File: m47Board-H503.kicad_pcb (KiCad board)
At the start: 4 copper layers, 40 x 34 mm, 42 parts, among them J1 USB_C_Receptacle_USB2.0_16P, J3 Conn_01x15_Pin, J4 Conn_01x10_Pin, J5 Conn_01x15_Pin, SW1 SW_Push, SW2 SW_Push, SW3 SW_Push, U1 AP2114H-3.3TRG1, U2 STM32H503CBTx, U3 USBLC6-2SC6, Y1 CX3225FB16000F0FZZH1 16MHz, Y2 ABS07-32.768KHZ-T

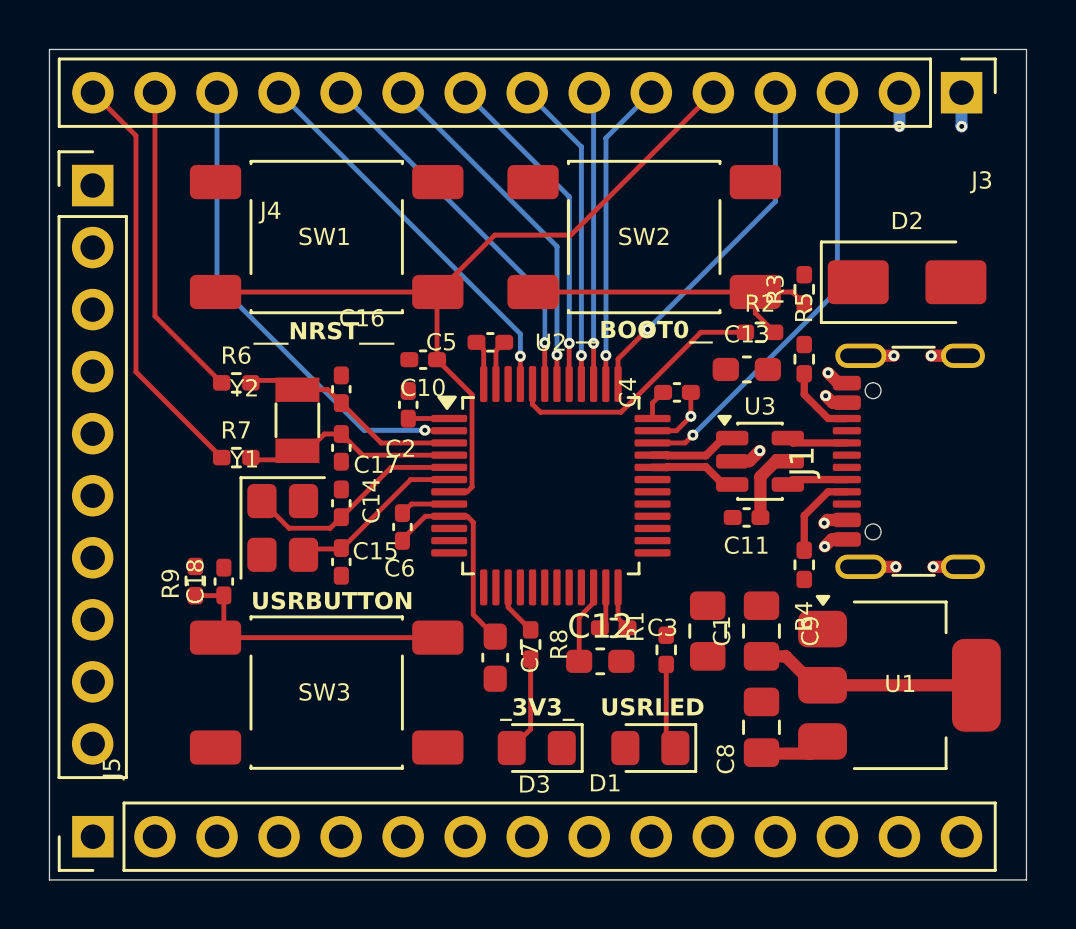
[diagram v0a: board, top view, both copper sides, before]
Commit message: Route tracks
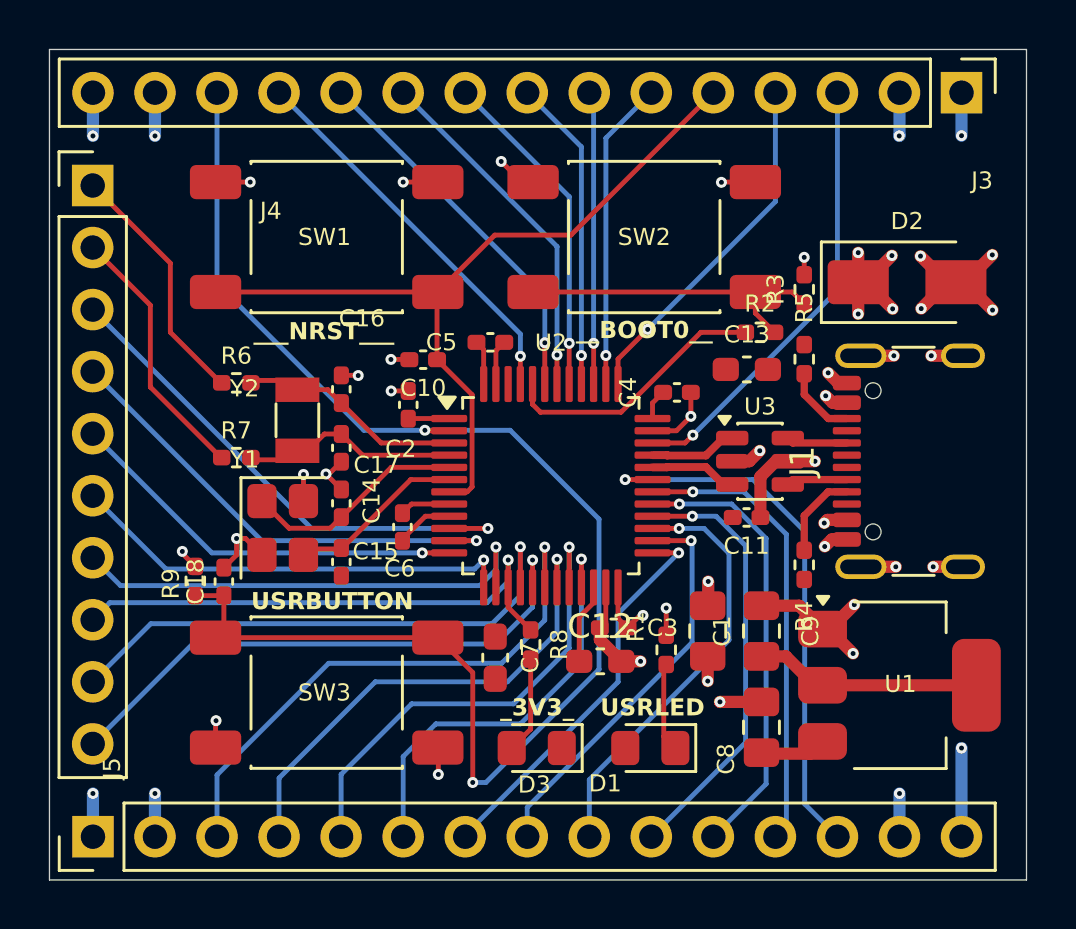
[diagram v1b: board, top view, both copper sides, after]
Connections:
- J3 pad 14: Net-(J3-Pin_14) -> GND
- J3 pad 15: Net-(J3-Pin_15) -> +3.3V
- J4 pad 1: unconnected-(J4-Pin_1-Pad1) -> Net-(J4-Pin_1)
- J4 pad 10: unconnected-(J4-Pin_10-Pad10) -> /PA7
- J4 pad 2: unconnected-(J4-Pin_2-Pad2) -> Net-(J4-Pin_2)
- J4 pad 3: unconnected-(J4-Pin_3-Pad3) -> /PA0
- J4 pad 4: unconnected-(J4-Pin_4-Pad4) -> /PA1
- J4 pad 5: unconnected-(J4-Pin_5-Pad5) -> /PA2
- J4 pad 6: unconnected-(J4-Pin_6-Pad6) -> /PA3
- J4 pad 7: unconnected-(J4-Pin_7-Pad7) -> /PA4
- J4 pad 8: unconnected-(J4-Pin_8-Pad8) -> /PA5
- J4 pad 9: unconnected-(J4-Pin_9-Pad9) -> /PA6
- J5 pad 1: unconnected-(J5-Pin_1-Pad1) -> +3.3V
- J5 pad 10: unconnected-(J5-Pin_10-Pad10) -> /PB15
- J5 pad 11: unconnected-(J5-Pin_11-Pad11) -> /PA8
- J5 pad 12: unconnected-(J5-Pin_12-Pad12) -> /PA9
- J5 pad 13: unconnected-(J5-Pin_13-Pad13) -> /PA10
- J5 pad 14: unconnected-(J5-Pin_14-Pad14) -> GND
- J5 pad 15: unconnected-(J5-Pin_15-Pad15) -> VBUS
- J5 pad 2: unconnected-(J5-Pin_2-Pad2) -> GND
- J5 pad 3: unconnected-(J5-Pin_3-Pad3) -> /PB0
- J5 pad 4: unconnected-(J5-Pin_4-Pad4) -> /PB1
- J5 pad 5: unconnected-(J5-Pin_5-Pad5) -> /PB2
- J5 pad 6: unconnected-(J5-Pin_6-Pad6) -> /PB10
- J5 pad 7: unconnected-(J5-Pin_7-Pad7) -> /PB12
- J5 pad 8: unconnected-(J5-Pin_8-Pad8) -> /PB13
- J5 pad 9: unconnected-(J5-Pin_9-Pad9) -> /PB14
- R6 pad 2: Net-(J3-Pin_14) -> Net-(J4-Pin_1)
- R7 pad 2: Net-(J3-Pin_15) -> Net-(J4-Pin_2)
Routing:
- net GND: track 18.4 -> 57.9 mm, vias 9 -> 33
- net /PC13: track 32.0 -> 60.4 mm, vias 1 -> 2
- net /PA7: track 0.00 -> 23.4 mm, vias 0 -> 1
- net /PB0: track 0.00 -> 23.2 mm, vias 0 -> 1
- net /PA6: track 0.00 -> 22.6 mm, vias 0 -> 1
- net /PA10: track 0.00 -> 22.4 mm, vias 0 -> 1
- net /PA0: track 0.00 -> 21.5 mm, vias 0 -> 1
- net /PB1: track 0.00 -> 20.4 mm, vias 0 -> 1
- net /PA4: track 0.00 -> 19.8 mm, vias 0 -> 1
- net /PB2: track 0.00 -> 19.8 mm, vias 0 -> 1
- net /PA1: track 0.00 -> 19.7 mm, vias 0 -> 1
- net /PA5: track 2.12 -> 21.8 mm, vias 0 -> 1
- net /PA9: track 0.00 -> 18.8 mm, vias 0 -> 1
- net /PA3: track 0.00 -> 18.5 mm, vias 0 -> 1
- net /PA8: track 0.00 -> 18.3 mm, vias 0 -> 1
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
